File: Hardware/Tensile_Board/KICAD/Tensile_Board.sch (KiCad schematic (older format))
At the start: 27 parts, among them J1 Conn_02x05_Odd_Even, J11 Screw_Terminal_01x04, J2 Conn_02x05_Odd_Even, J3 Conn_02x05_Odd_Even, J4 Conn_02x05_Odd_Even, J5 Micro_SD_Card, J6 Main_Power, J9 Grounding, U2 AMS1117-3.3, U20 APM4953, U3 DS3231M

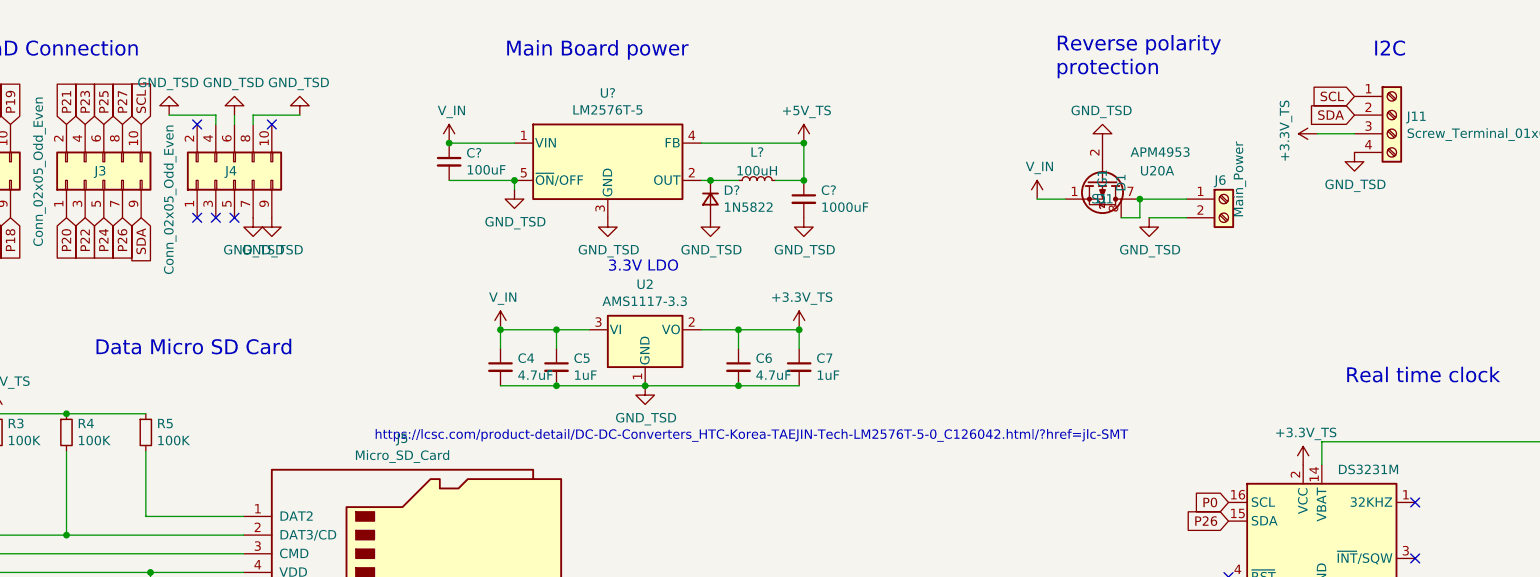
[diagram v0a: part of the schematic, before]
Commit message: groundwork for p2
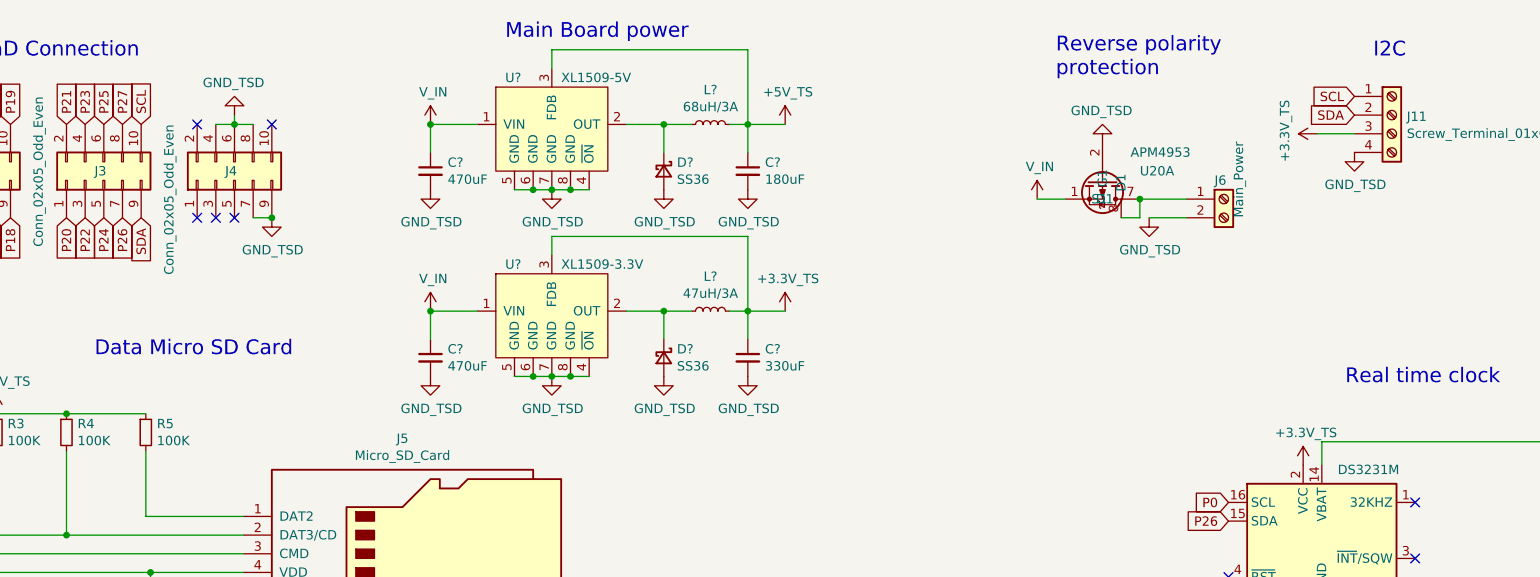
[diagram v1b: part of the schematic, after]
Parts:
- removed C4, C6: 4.7uF, Capacitor_SMD:C_0805_2012Metric, symbol Device:C_Small
- removed C5, C7: 1uF, Capacitor_SMD:C_0603_1608Metric, symbol Device:C_Small
- removed C?: 100uF, Capacitor_SMD:C_0805_2012Metric, symbol Device:C_Small
- removed C?: 1000uF, Capacitor_SMD:C_0805_2012Metric, symbol Device:C_Small
- removed D?: 1N5822, symbol Device:D_Small
- removed L?: 100uH, symbol Device:L_Small
- removed U2: AMS1117-3.3, Package_TO_SOT_SMD:SOT-223-3_TabPin2, symbol Regulator_Linear:AMS1117-3.3
- removed U?: LM2576T-5, Package_TO_SOT_THT:TO-220-5_Vertical, symbol Regulator_Switching:LM2576T-5
- added C? (x2): 470uF, symbol Device:C_Small
- added C?: 180uF, symbol Device:C_Small
- added C?: 330uF, symbol Device:C_Small
- added D? (x2): SS36, symbol Device:D_Schottky_Small
- added L?: 68uH/3A, symbol Device:L_Small
- added L?: 47uH/3A, symbol Device:L_Small
- added U?: XL1509-5V, symbol Tensile_Board:XL1509
- added U?: XL1509-3.3V, symbol Tensile_Board:XL1509
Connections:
- net +3V3_TS: now also C?.1, L?.2, U?.3 (FDB)
- net +5V_TS: now also C?.1, L?.2, U?.3 (FDB)
- net GND_TSD: now also C?.2, C?.2, C?.2, C?.2, D?.2 (A), D?.2 (A), U?.4 (~ON), U?.4 (~ON), U?.5 (GND), U?.5 (GND), U?.6 (GND), U?.6 (GND), U?.7 (GND), U?.7 (GND), U?.8 (GND), U?.8 (GND)
- net V_IN: now also C?.1, C?.1, U?.1 (VIN), U?.1 (VIN)
- new net: D?.1 (K), L?.1, U?.2 (OUT) (x2)
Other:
- note removed: "3.3V LDO"
- note removed: "https://lcsc.com/product-detail/DC-DC-Converters_HTC-Korea-TAEJIN-Tech-LM2576T-5-0_C126042.html/?href=jlc-SMT"
